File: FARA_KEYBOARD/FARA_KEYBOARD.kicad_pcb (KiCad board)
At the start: 2 copper layers, 72.2 x 65.6 mm, 36 parts, among them J1 Conn_01x07_Pin, J10 Conn_01x02, J11 Screw_Terminal_01x02, J12 Screw_Terminal_01x02, J13 Conn_01x02, J2 Conn_01x20, J3 Conn_01x20, J4 Conn_01x04, J5 Conn_01x03, J6 Conn_01x03, J7 Conn_01x03, J8 Conn_01x03, J9 Conn_01x03, Q1 AO3400A, Q2 AO3400A, Q3 AO3400A, SW1 SW_Push, SW2 SW_Push, SW3 SW_Push, SW4 SW_Push, SW5 SW_Push, SW6 SW_Push, U1 Raspberri_Pi_Pico

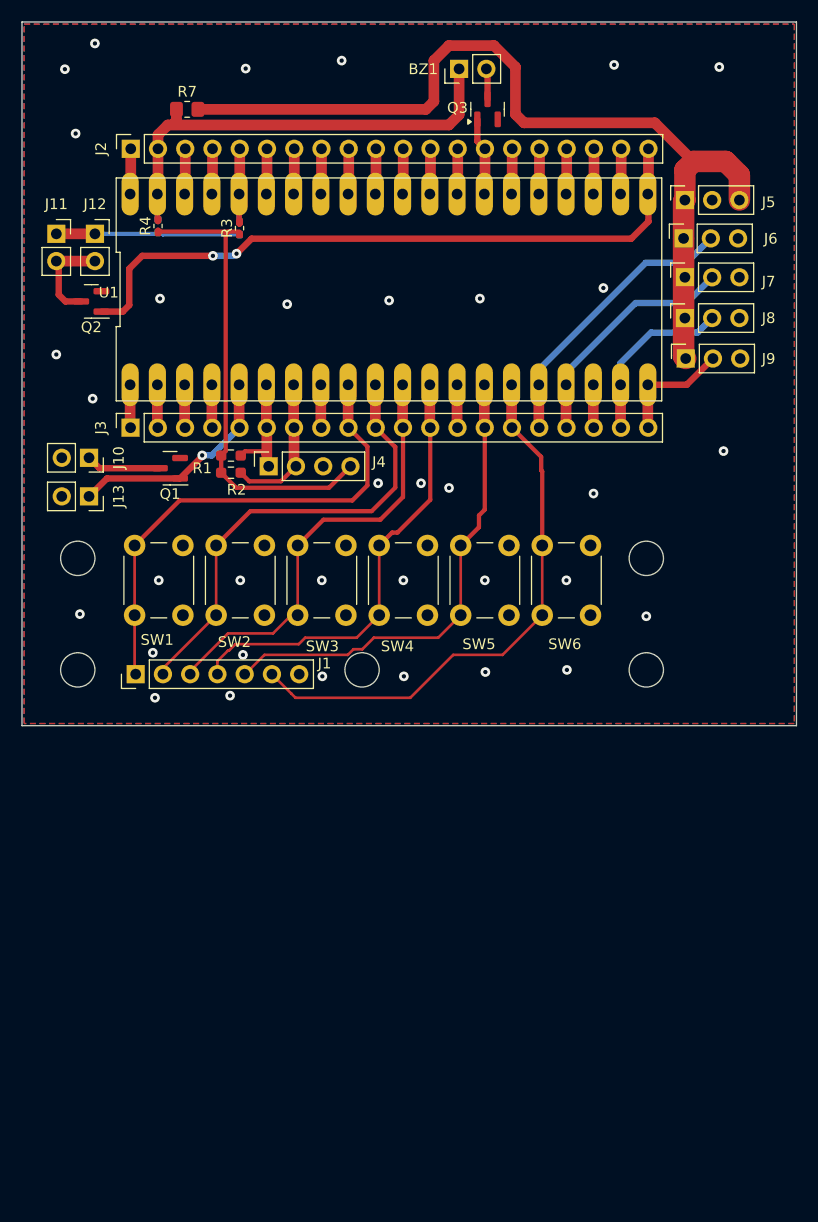
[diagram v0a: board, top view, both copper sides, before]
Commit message: v0.6 seems 2B ready
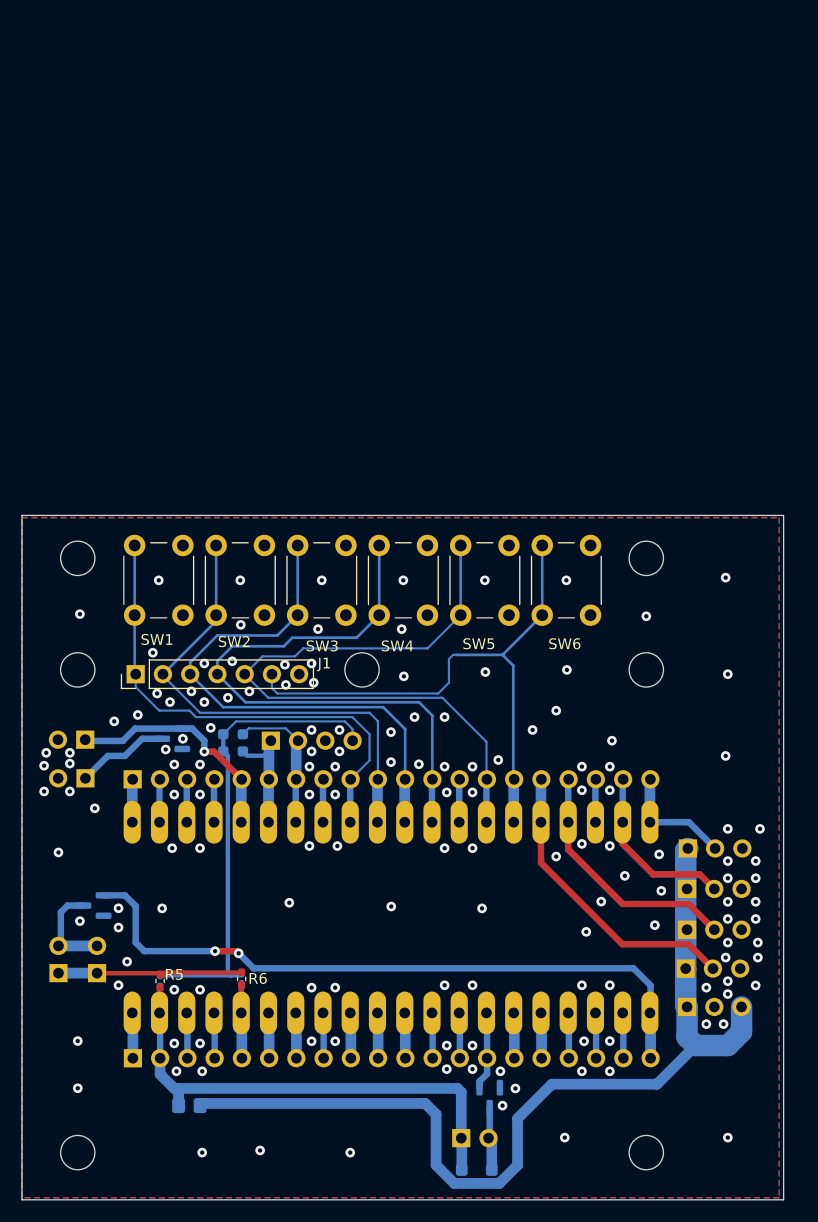
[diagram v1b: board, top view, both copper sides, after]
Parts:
- added D1: PMEG3010CEH, Diode_SMD:D_SOD-123F, B.Cu at (89.4, 140.6)
- added REF**: MountingHole_3.2mm_M3, MountingHole:MountingHole_3.2mm_M3, F.Cu at (52.2, 139.0)
- added REF**: MountingHole_3.2mm_M3, MountingHole:MountingHole_3.2mm_M3, F.Cu at (105.2, 139.0)
- BZ1, J10, J11, J12, J13, J2, J3, J4, J5, J6, J7, J8, J9, Q1, Q2, Q3, R1, R2, R3, R4, R7, U1: moved to B.Cu
- R5, R6: moved to F.Cu
- moved BZ1 99.7 mm to (88.0, 137.7), turned to -90 degrees
- moved R7 92.9 mm to (62.6, 134.6)
- moved Q3 92.1 mm to (90.6, 133.9), turned to -90 degrees
- moved J2 84.8 mm to (57.3, 130.2), turned to -90 degrees
- moved J5 75.2 mm to (109.0, 125.4), turned to -90 degrees
- moved R4 70.4 mm to (59.9, 123.0), turned to -90 degrees
- moved R5 70.4 mm to (59.9, 123.0), turned to -90 degrees
- moved R3 70.0 mm to (67.5, 122.8), turned to -90 degrees
- moved R6 70.0 mm to (67.5, 122.8), turned to -90 degrees
- moved J11 68.9 mm to (50.4, 122.3)
- moved J12 68.9 mm to (54.0, 122.3)
- moved J6 68.1 mm to (108.9, 121.8), turned to -90 degrees
- moved J7 60.8 mm to (109.0, 118.2), turned to -90 degrees
- moved U1 58.6 mm to (81.4, 117.1)
- moved Q2 56.3 mm to (53.7, 116.0)
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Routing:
- net SW5: track 44.8 -> 62.3 mm
- net SW4: track 41.8 -> 56.2 mm
- net SW3: track 41.1 -> 51.0 mm
- net Net-(BZ1-+): track 2.88 -> 5.97 mm
- net SW2: track 43.4 -> 46.4 mm
- net +5V: track 45.0 -> 47.7 mm
- net VPP: track 83.9 -> 86.0 mm
- net Net-(J10-Pin_1): track 7.02 -> 8.68 mm
- net SW6: track 52.0 -> 53.6 mm
- net STRIP0: track 26.5 -> 27.9 mm
- net LEDS: track 20.8 -> 21.7 mm
- net STRIP1: track 22.5 -> 23.3 mm
- net GND: vias 35 -> 148
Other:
- board size 72.2 x 65.6 mm -> 71 x 63.8 mm
